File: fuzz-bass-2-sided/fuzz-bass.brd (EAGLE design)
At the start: 59.7 x 39.4 mm, 0 parts

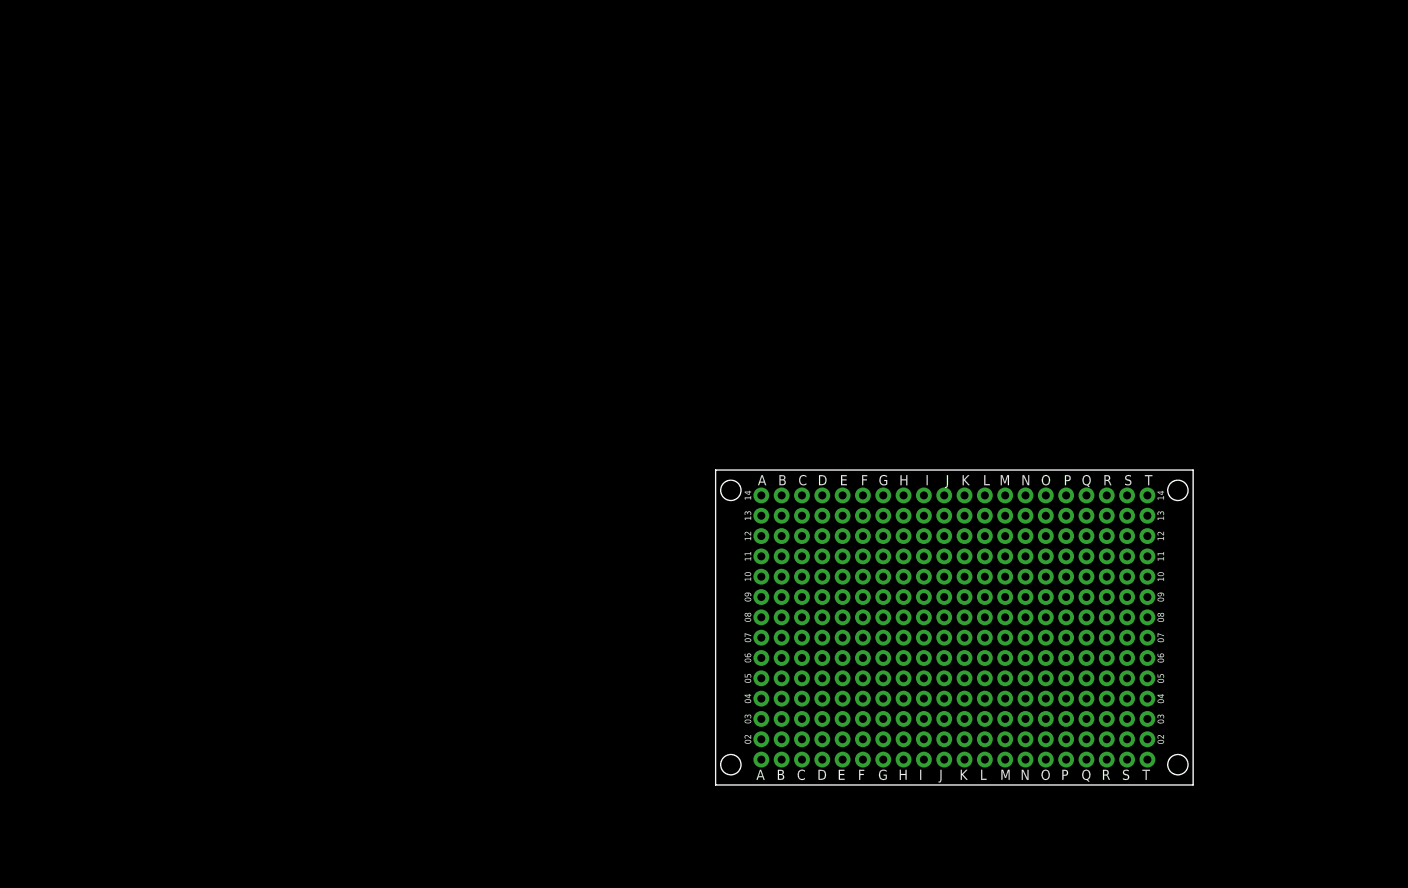
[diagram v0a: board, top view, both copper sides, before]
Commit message: Add pedal library to quickly access parts I have.
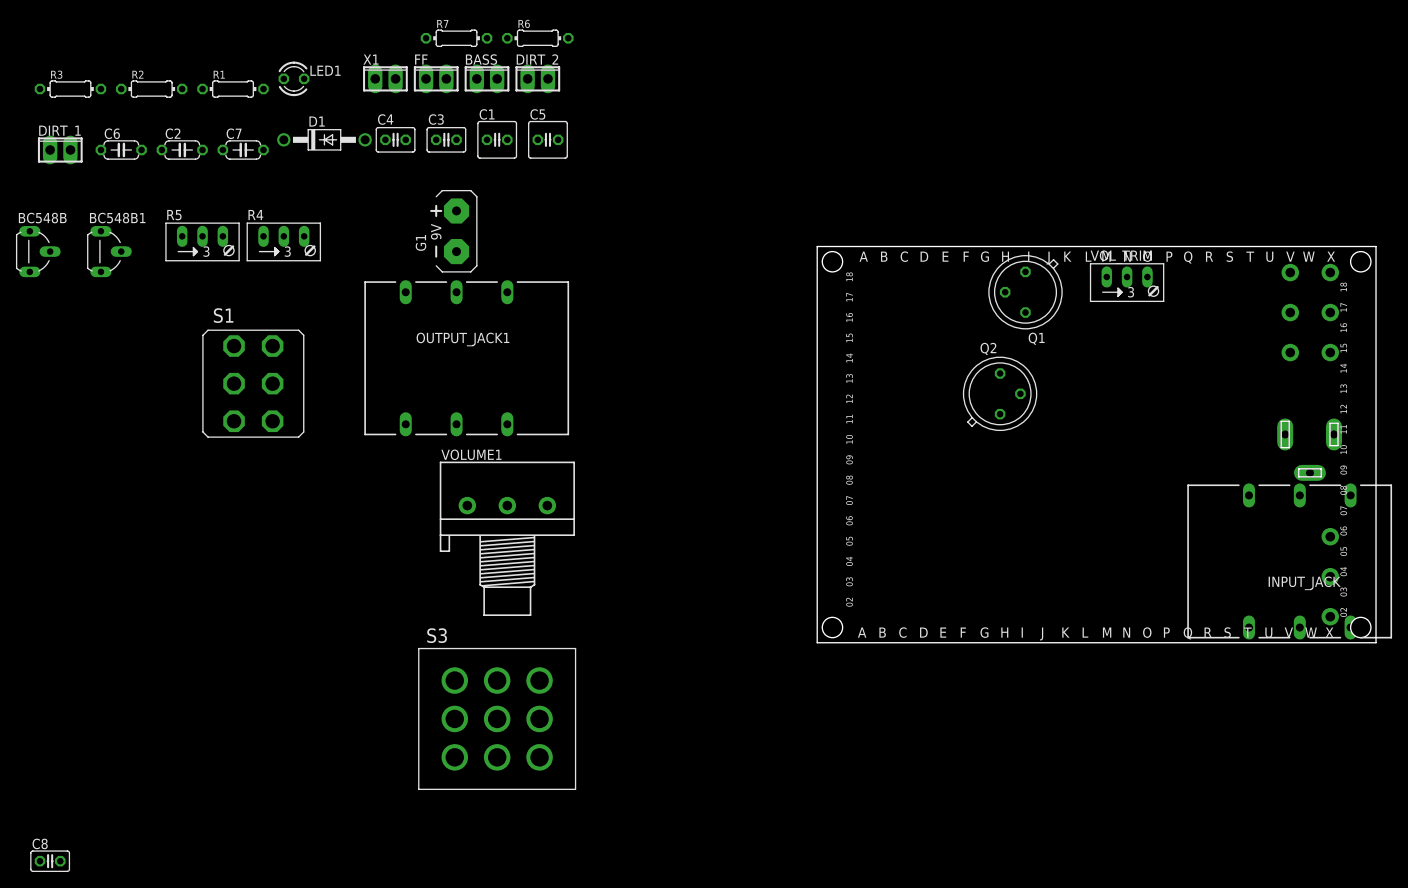
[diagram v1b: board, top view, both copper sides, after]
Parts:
- added BASS, DIRT_1, DIRT_2, FF, X1: (no value), con-phoenix-254:2POL254
- added BC548B, BC548B1: (no value), transistor:TO92L
- added C1: 2.2u, adafruit:C025-050X050
- added C2: 0.1u, rcl:C050-024X044
- added C3, C4: 20u, rcl:C025-030X050
- added C5: 0.22u, adafruit:C025-050X050
- added C6: 0.22u, rcl:C050-024X044
- added C7: 0.001u, rcl:C050-024X044
- added C8: (no value), rcl:C025-025X050
- added D1: 1N4942, diode:DO41-10
- added DIRT: 1k, pot:3RP/1610G
- added G1: AB9V, battery:AB9V
- added INPUT_JACK, OUTPUT_JACK1: JACK6.35MM, jack-eagle:JACK6.35MM
- added J1: (no value), con-jack:DCJ0303
- added LED1: (no value), led:LED3MM
- added Q1, Q2: 2N4036, transistor-pnp:TO5
- added R1: 33k, rcl:0204/7
- added R2: 8.2k, rcl:0204/7
- added R3: 470, rcl:0204/7
- added R4, R5: 200k, pot:RJ9W
- added R6: 100k, rcl:0204/7
- added R7: 1M, rcl:0204/7
- added S1: (no value), switch:M9040P2
- added S3: 3PDT, switch:3PDT
- added VOLUME, VOLUME1: 500k, pot:3RP/1610N
- added VOL_TRIM: 100k, pot:RJ9W
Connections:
- new net +9V: C3.1, DIRT.1-1, DIRT_1.2, G1.+, Q1.1, R5.A, R5.S, S3.5, X1.1
- new net BASS_DIRT_IN: BC548B1.1, DIRT.2-3, DIRT_2.1
- new net BASS_IN: BASS.1, C5.2, S1.3
- new net BASS_OUT: BASS.2, S1.6, VOL_TRIM.S
- new net FACE_DIRT_IN: DIRT.1-3, DIRT_1.1, Q2.1, R4.A, R4.S
- new net FUZZED_OUTPUT: S3.9, VOLUME.2
- new net FUZZ_FACE_IN: C1.2, FF.1, S1.1
- new net FUZZ_FACE_OUT: C2.2, FF.2, S1.4
- new net GND: DIRT.2-1, DIRT.2-2, INPUT_JACK.0, INPUT_JACK.3, LED1.K, OUTPUT_JACK1.0, OUTPUT_JACK1.3, R1.2, R3.2, R7.1, VOLUME.1, VOL_TRIM.A, X1.2
- new net INPUT: C7.1, INPUT_JACK.2, R7.2, S3.2, VOLUME1.1
- new net N$1: Q2.3, R2.1
- new net N$10: LED1.A, R6.2
- new net N$11: BC548B.2, C5.1, D1.C
- new net N$12: C4.1, VOL_TRIM.E
- new net N$13: C6.1, VOLUME1.2, VOLUME1.3
- new net N$14: S3.1, S3.7
- new net N$15: G1.-, INPUT_JACK.1
- new net N$16: S1.5, VOLUME.3
- new net N$3: C1.1, Q1.2, R4.E
- new net N$4: Q1.3, Q2.2, R1.1
- new net N$5: C3.2, DIRT.1-2
- new net N$6: C2.1, R2.2, R3.1
- new net N$7: BC548B.1, BC548B1.2
- new net N$8: BC548B.3, BC548B1.3, C4.2, D1.A, R5.E
- new net N$9: R6.1, S3.6
- new net OUTPUT: OUTPUT_JACK1.2, S3.8
- new net TONE_INPUT: S3.3
- new net TONE_OUTPUT: C6.2, C7.2, S1.2
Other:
- board size 59.7 x 39.4 mm -> 69.9 x 49.5 mm
- board text added: "15"
- board text added: "16"
- board text added: "17"
- board text added: "18"
- board text added: "U"
- board text added: "V"
- board text added: "W"
- board text added: "X"
